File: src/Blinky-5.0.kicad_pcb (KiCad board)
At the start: 2 copper layers, 25 x 18 mm, 8 parts, among them SW1 SW_SPDT, U1 7555

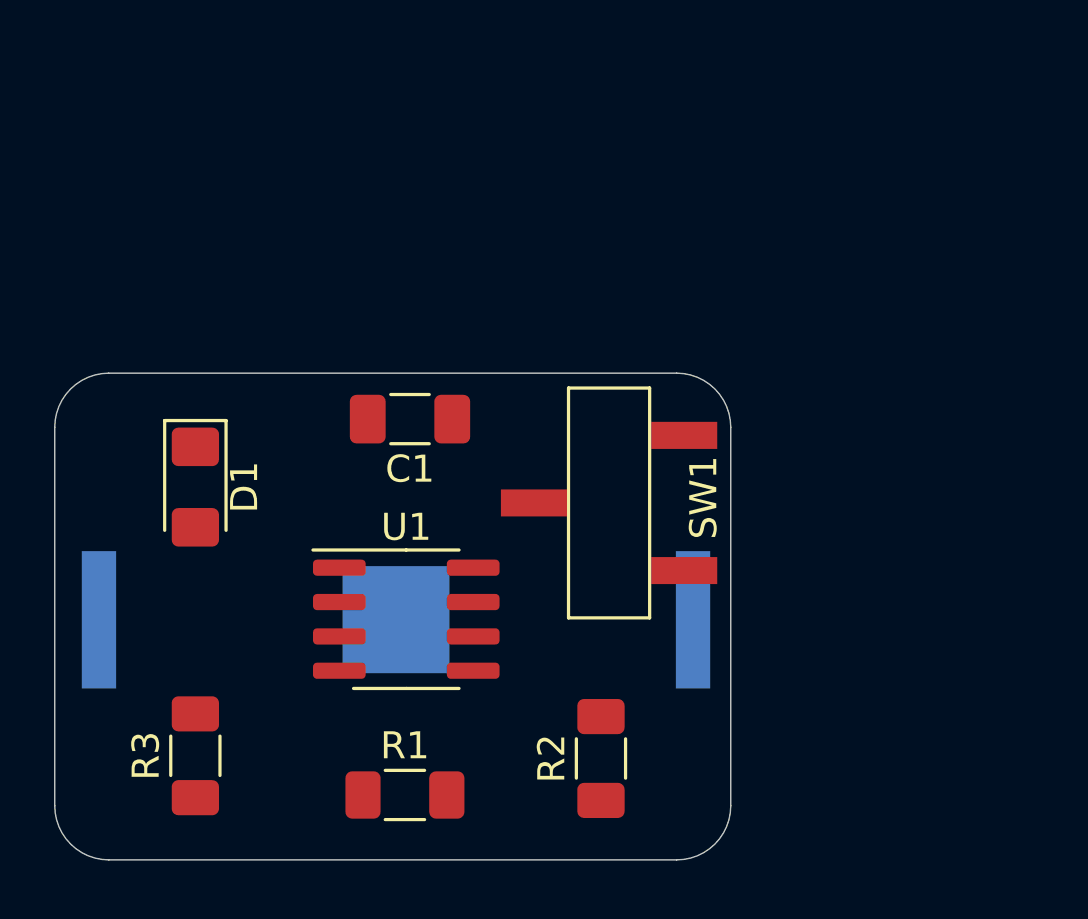
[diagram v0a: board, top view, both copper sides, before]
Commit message: Add some changes and finish layout
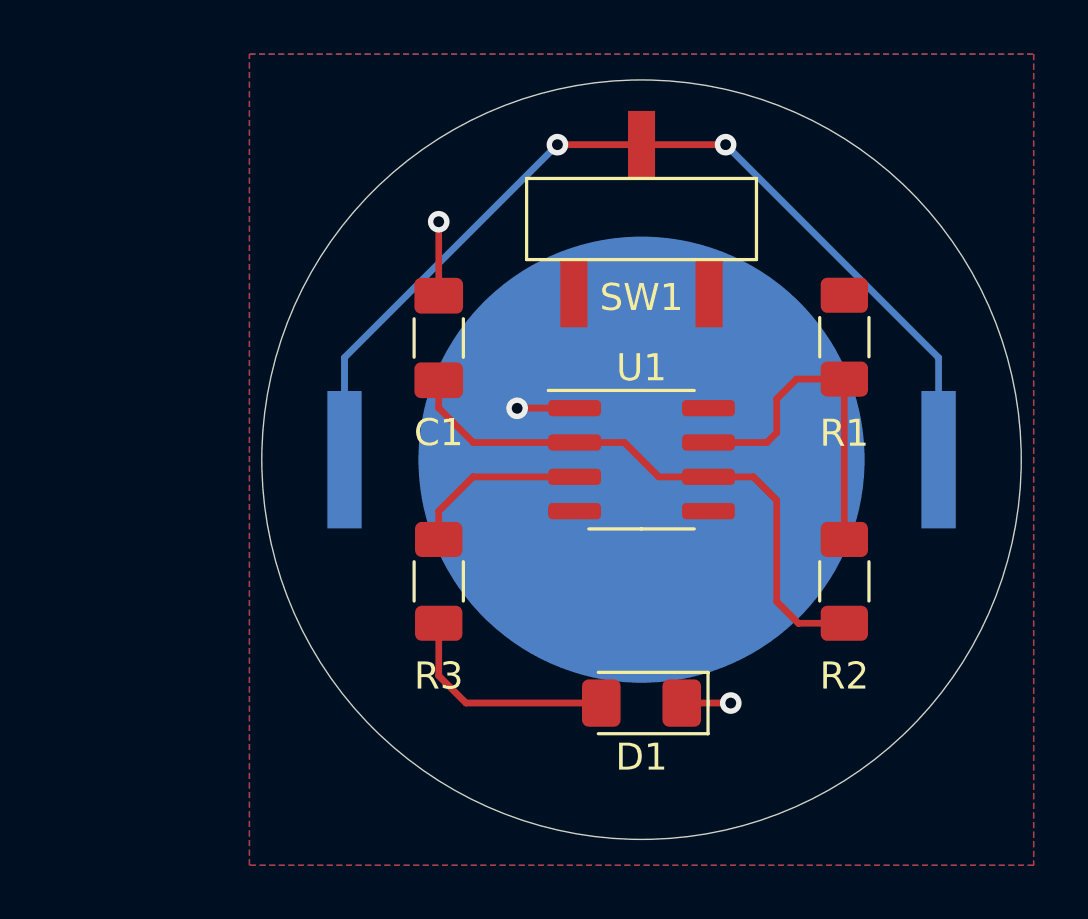
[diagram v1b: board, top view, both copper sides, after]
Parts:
- R3: value 1k -> 150
- moved R1 23.5 mm to (166.0, 90.5), turned to 270 degrees
- moved D1 18.3 mm to (158.5, 104.0), turned to 180 degrees
- moved R2 11.1 mm to (166.0, 99.5), turned to 270 degrees
- moved R3 11.1 mm to (151.0, 99.5), turned to 270 degrees
- moved BT1 10.8 mm to (158.5, 95.0)
- moved SW1 10.6 mm to (158.5, 86.1), turned to 0 degrees
- moved U1 10.5 mm to (158.5, 95.0)
- moved C1 3.18 mm to (151.0, 90.5), turned to 90 degrees
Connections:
- net VCC renamed VDD
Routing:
- net Net-(BT1-Pad1): track 0.00 -> 36.0 mm, vias 0 -> 2
- net Net-(C1-Pad1): track 0.00 -> 21.5 mm
- net Net-(R1-Pad2): track 0.00 -> 12.7 mm
- net Net-(D1-Pad2): track 0.00 -> 8.37 mm
- net GND: track 0.00 -> 6.68 mm, vias 0 -> 3
- net Net-(R3-Pad1): track 0.00 -> 6.60 mm
- added copper zone on B.Cu, net GND
- added copper zone on F.Cu, net VDD
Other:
- board size 25 x 18 mm -> 28.1 x 28.1 mm
- rule pad_to_mask_clearance: 0 -> 0.0508
- rule trace_min: 0.2 -> 0.000152
- rule via_min_size: 0.4 -> 0.000508
